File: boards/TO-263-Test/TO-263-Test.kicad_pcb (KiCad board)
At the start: 2 copper layers, 43.2 x 26.7 mm, 3 parts, among them J1 Conn_01x02, J2 Conn_01x02

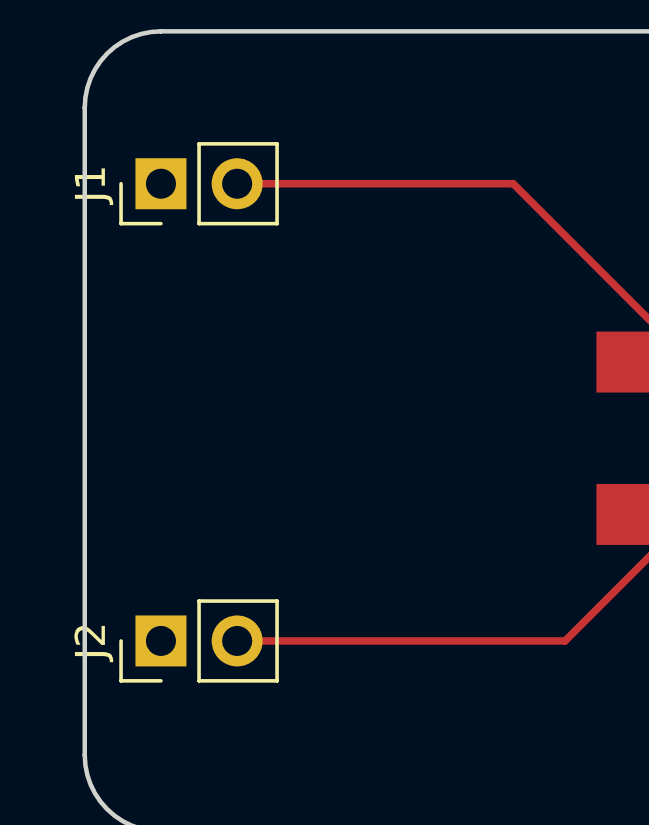
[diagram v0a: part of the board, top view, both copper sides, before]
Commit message: Adding changes to the TO-263 Test board
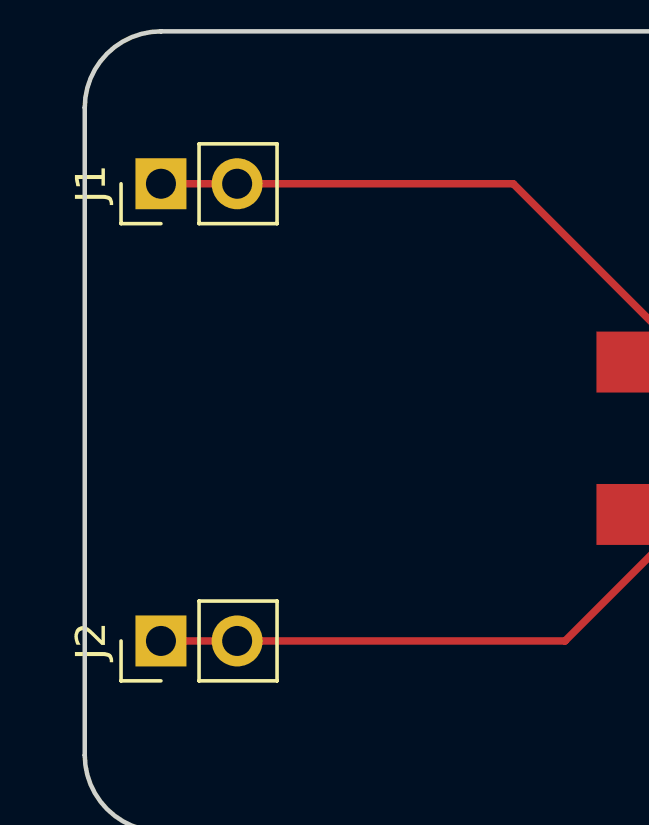
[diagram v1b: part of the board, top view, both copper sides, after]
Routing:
- net Net-(J2-Pad1): track 16.4 -> 18.9 mm
- net Net-(J1-Pad1): track 17.1 -> 19.6 mm
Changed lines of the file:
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@@
   (general
     (links 4)
-    (no_connects 0)
-    (area 119.304999 91.364999 162.635001 118.185001)
+    (no_connects 2)
+    (area 118.442381 90.01 162.635001 118.185001)
     (thickness 1.6)
     (drawings 10)
-    (tracks 6)
+    (tracks 8)
     (zones 0)
     (modules 3)
@@
   (gr_arc (start 121.92 115.57) (end 121.92 118.11) (angle 90) (layer Edge.Cuts) (width 0.15))
   (gr_arc (start 121.92 93.98) (end 119.38 93.98) (angle 90) (layer Edge.Cuts) (width 0.15))
+  (segment (start 121.92 96.52) (end 124.46 96.52) (width 0.25) (layer F.Cu) (net 1))
   (segment (start 124.46 96.52) (end 133.6635 96.52) (width 0.25) (layer F.Cu) (net 1))
   (segment (start 133.6635 96.52) (end 138.3411 101.1976) (width 0.25) (layer F.Cu) (net 1))
   (segment (start 138.3411 101.1976) (end 138.3411 102.4636) (width 0.25) (layer F.Cu) (net 1))
+  (segment (start 121.92 111.76) (end 124.46 111.76) (width 0.25) (layer F.Cu) (net 2))
   (segment (start 124.46 111.76) (end 135.3907 111.76) (width 0.25) (layer F.Cu) (net 2))
   (segment (start 135.3907 111.76) (end 138.3411 108.8096) (width 0.25) (layer F.Cu) (net 2))
